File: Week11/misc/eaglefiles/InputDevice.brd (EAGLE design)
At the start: 46.4 x 29.2 mm, 9 parts, among them J1 AVRISPSMD

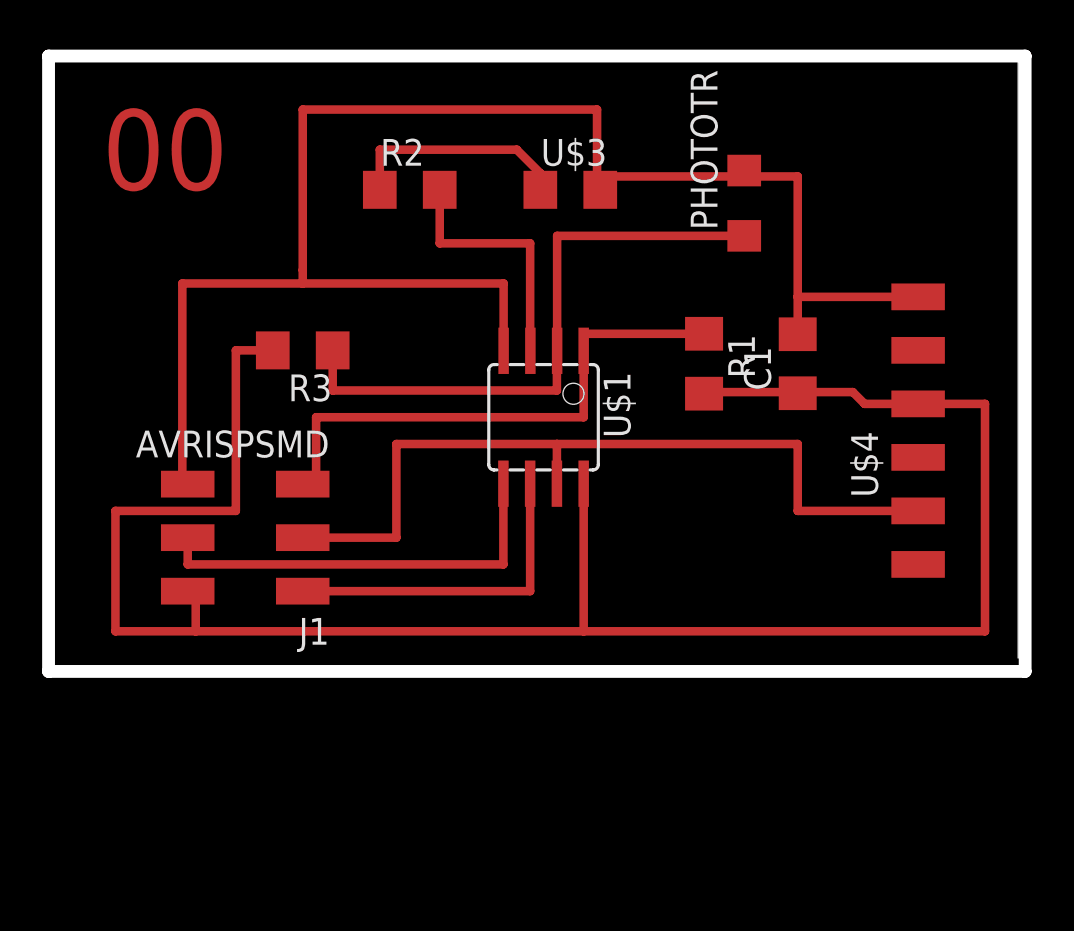
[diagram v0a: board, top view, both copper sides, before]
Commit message: refinements
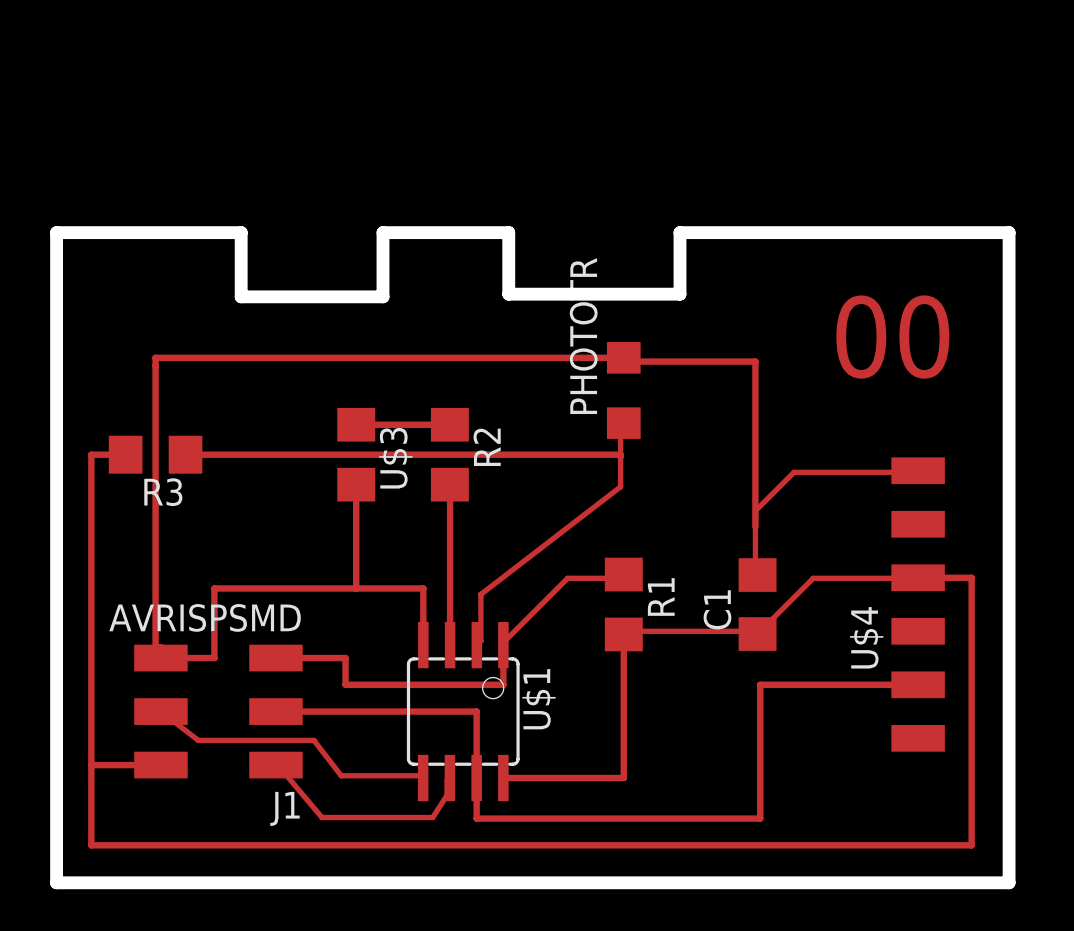
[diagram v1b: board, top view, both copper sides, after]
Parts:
- moved U$3 16.2 mm to (14.0, 19.8), turned to 270 degrees
- moved U$1 14.5 mm to (19.1, 7.62)
- moved R2 12.7 mm to (18.4, 19.8), turned to 270 degrees
- moved R1 12.0 mm to (26.7, 12.7)
- moved C1 11.6 mm to (33.0, 12.7)
- moved PHOTOTR 10.6 mm to (26.7, 22.9)
- moved R3 8.56 mm to (4.45, 19.8)
- moved J1 8.35 mm to (7.62, 7.62)
- moved U$4 8.25 mm to (40.6, 12.7)
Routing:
- net VCC: track 96.7 -> 108.2 mm
- net GND: track 77.6 -> 86.2 mm
- net N$1: track 10.8 -> 4.44 mm
- net MOSI: track 20.1 -> 13.8 mm
- net PA: track 28.8 -> 34.8 mm
- net MISO: track 16.5 -> 10.7 mm
- net RST: track 26.8 -> 21.1 mm
- net LED: track 11.9 -> 7.63 mm
- net SCK: track 38.7 -> 41.9 mm
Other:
- board size 46.4 x 29.2 mm -> 45.2 x 30.9 mm
